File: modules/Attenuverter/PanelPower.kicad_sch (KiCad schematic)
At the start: 26 parts, among them J1 WQP-PJ398, J10 Conn_Front, J11 Conn_Back, J2 WQP-PJ398, J3 WQP-PJ398, J4 WQP-PJ398, J9 Conn_Eurorack_Pwr_10, U1 TL074, U2 TL074, U3 LM4040, U4 LM4040

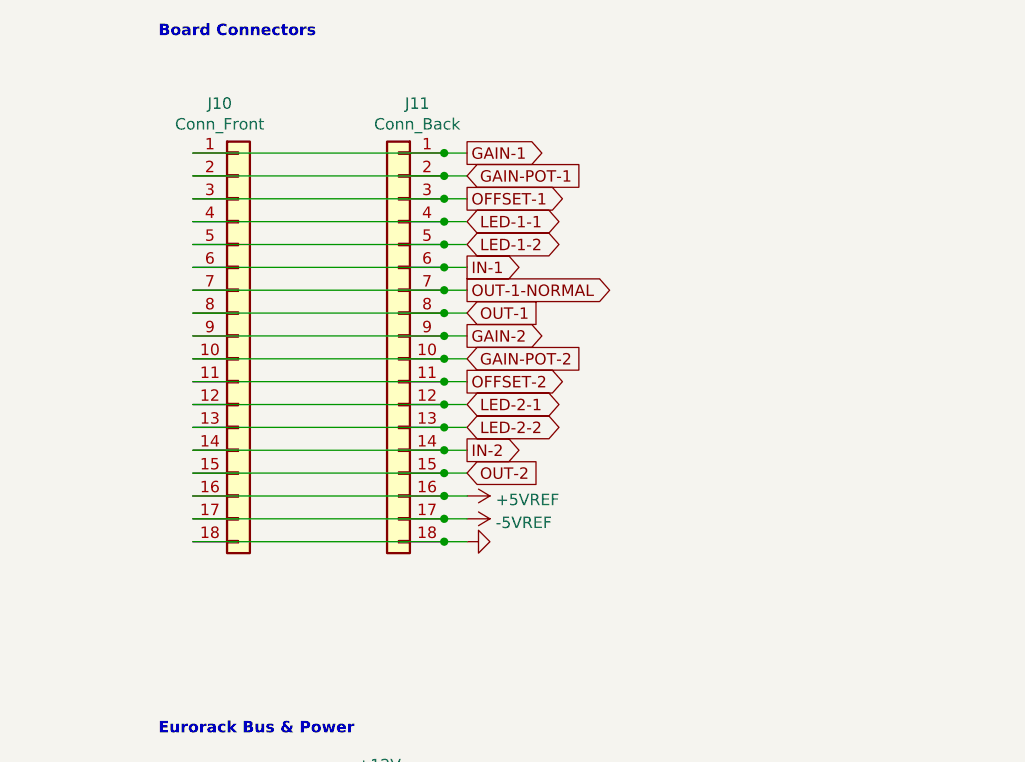
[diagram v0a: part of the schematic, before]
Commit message: Attenuverter - wip
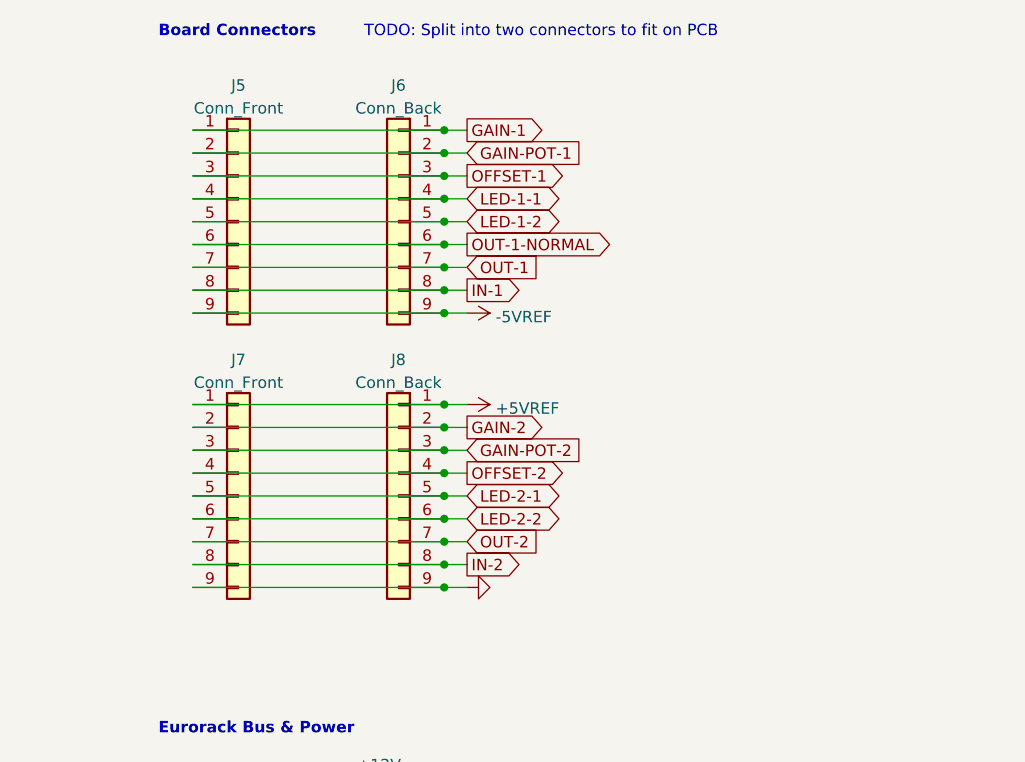
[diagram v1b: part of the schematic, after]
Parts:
- added J7: Conn_Front, Connector_PinSocket_2.54mm:PinSocket_1x09_P2.54mm_Vertical, symbol Connector_Generic:Conn_01x09
- added J8: Conn_Back, Connector_PinHeader_2.54mm:PinHeader_1x09_P2.54mm_Horizontal, symbol Connector_Generic:Conn_01x09
- J5: renamed from J10; footprint Connector_PinSocket_2.54mm:PinSocket_1x18_P2.54mm_Vertical -> Connector_PinSocket_2.54mm:PinSocket_1x09_P2.54mm_Vertical; symbol Connector_Generic:Conn_01x18 -> Connector_Generic:Conn_01x09
- J6: renamed from J11; footprint Connector_PinHeader_2.54mm:PinHeader_1x18_P2.54mm_Horizontal -> Connector_PinHeader_2.54mm:PinHeader_1x09_P2.54mm_Horizontal; symbol Connector_Generic:Conn_01x18 -> Connector_Generic:Conn_01x09
- U3, U4: footprint -lmp-misc:TO-92-2_Wide -> -lmp-misc:TO-92-2_Inline
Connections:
- net +5VREF: now also J7.1 (Pin_1), J8.1 (Pin_1); no longer J5.16 (Pin_16), J6.16 (Pin_16)
- net -5VREF: now also J5.9 (Pin_9), J6.9 (Pin_9); no longer J5.17 (Pin_17), J6.17 (Pin_17)
- net GAIN-2: now also J7.2 (Pin_2), J8.2 (Pin_2); no longer J5.9 (Pin_9), J6.9 (Pin_9)
- net GAIN-POT-2: now also J7.3 (Pin_3), J8.3 (Pin_3); no longer J5.10 (Pin_10), J6.10 (Pin_10)
- net GND: now also J7.9 (Pin_9), J8.9 (Pin_9); no longer J5.18 (Pin_18), J6.18 (Pin_18)
- net IN-1: now also J5.8 (Pin_8), J6.8 (Pin_8); no longer J5.6 (Pin_6), J6.6 (Pin_6)
- net IN-2: now also J7.8 (Pin_8), J8.8 (Pin_8); no longer J5.14 (Pin_14), J6.14 (Pin_14)
- net LED-2-1: now also J7.5 (Pin_5), J8.5 (Pin_5); no longer J5.12 (Pin_12), J6.12 (Pin_12)
- net LED-2-2: now also J7.6 (Pin_6), J8.6 (Pin_6); no longer J5.13 (Pin_13), J6.13 (Pin_13)
- net OFFSET-2: now also J7.4 (Pin_4), J8.4 (Pin_4); no longer J5.11 (Pin_11), J6.11 (Pin_11)
- net OUT-1: now also J5.7 (Pin_7), J6.7 (Pin_7); no longer J5.8 (Pin_8), J6.8 (Pin_8)
- net OUT-1-NORMAL: now also J5.6 (Pin_6), J6.6 (Pin_6); no longer J5.7 (Pin_7), J6.7 (Pin_7)
- net OUT-2: now also J7.7 (Pin_7), J8.7 (Pin_7); no longer J5.15 (Pin_15), J6.15 (Pin_15)
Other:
- note added: "TODO: Split into two connectors to fit on PCB"
